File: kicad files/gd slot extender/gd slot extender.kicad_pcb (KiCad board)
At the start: 2 copper layers, 11 parts, among them J1 Card Edge, J2 Debug Header, J3 Sockety Socket Sock

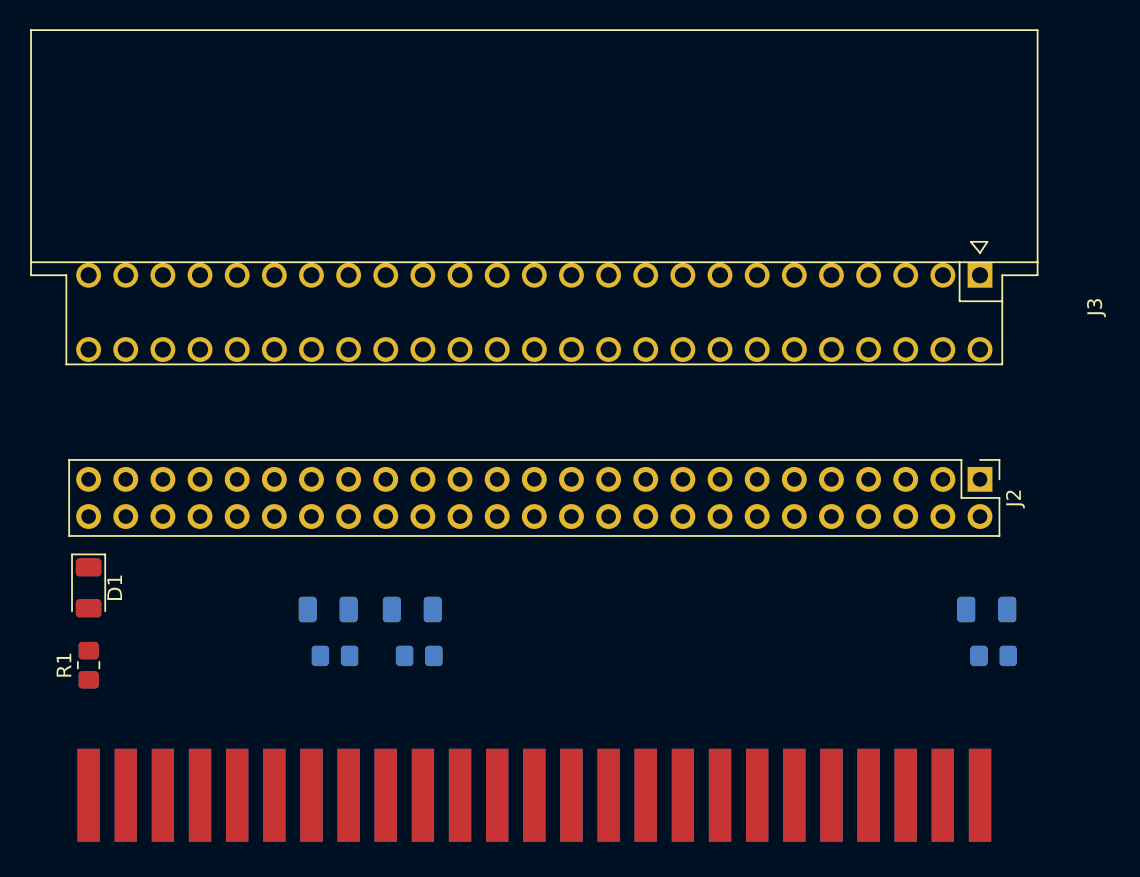
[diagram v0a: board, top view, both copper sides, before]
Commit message: rev1 ready for fab
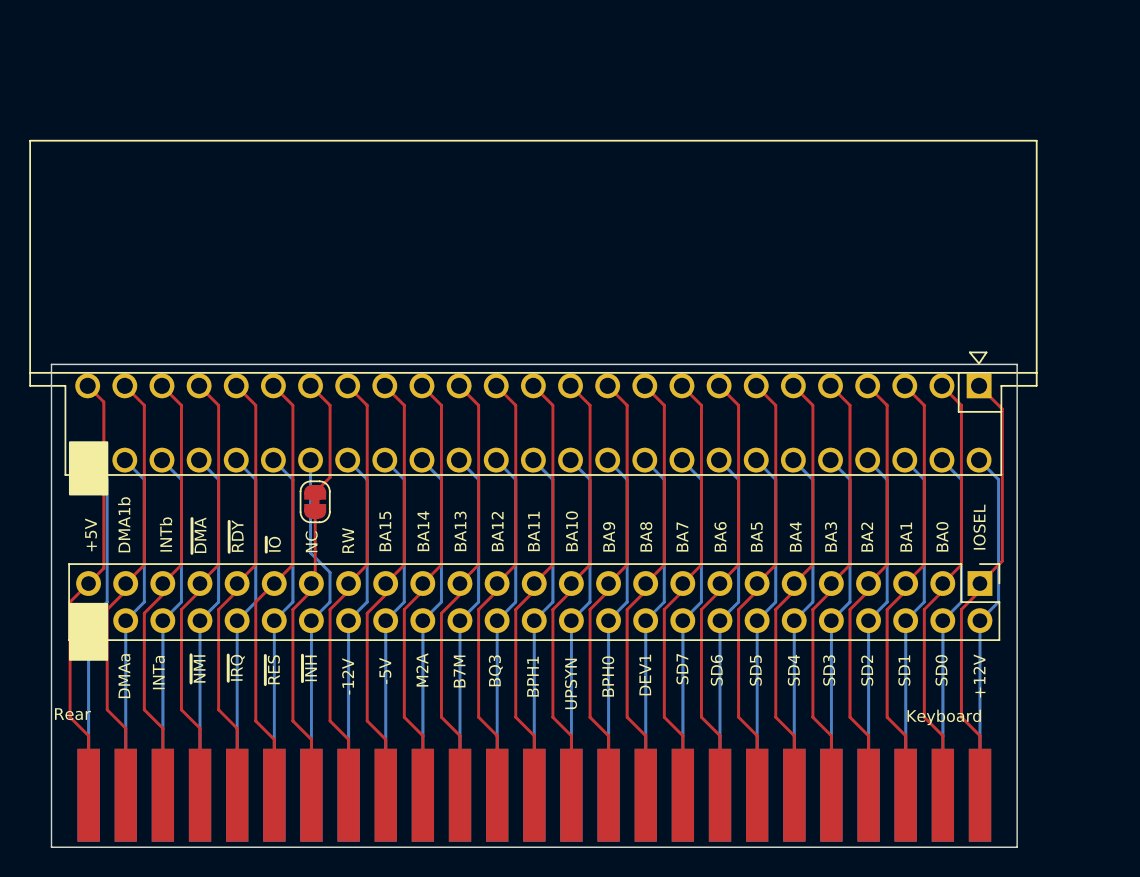
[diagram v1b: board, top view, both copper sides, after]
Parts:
- removed D1, D2, D3, D4: D_1206, LED_SMD:LED_1206_3216Metric
- removed R1, R2, R3, R4: 4k7, Resistor_SMD:R_0805_2012Metric_Pad1.20x1.40mm_HandSolder
- added JP1: Jumper_2_Bridged, Jumper:SolderJumper-2_P1.3mm_Bridged_RoundedPad1.0x1.5mm, F.Cu at (170.4, 106.9)
- moved J3 7.56 mm to (218.6, 102.1)
- moved J2 7.12 mm to (215.9, 112.5)
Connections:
- J1 pad 19: unconnected-(J1-Pad19) -> /NC
- J2 pad 19: unconnected-(J2-Pad19) -> /NC
- J3 pad 19: unconnected-(J3-Pad19) -> Net-(JP1-A)
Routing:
- net /~{IOSEL}: track 0.00 -> 30.3 mm
- net /~{DMA}: track 0.00 -> 30.1 mm
- net /RW: track 0.00 -> 30.1 mm
- net /BA9: track 0.00 -> 30.1 mm
- net /BA5: track 0.00 -> 30.1 mm
- net /BA2: track 0.00 -> 30.1 mm
- net /BA13: track 0.00 -> 30.1 mm
- net /~{RDY}: track 0.00 -> 30.1 mm
- net /BA15: track 0.00 -> 30.1 mm
- net /INTb: track 0.00 -> 30.1 mm
- net /BA8: track 0.00 -> 30.1 mm
- net /BA3: track 0.00 -> 30.1 mm
- net /BA12: track 0.00 -> 30.1 mm
- net /BA1: track 0.00 -> 30.1 mm
- net /BA7: track 0.00 -> 30.1 mm
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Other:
- board outline added: 66 x 33 mm
- board text added: "+12V"
- board text added: "+5V"
- board text added: "-12V"
- board text added: "-5V"
- board text added: "B7M"
- board text added: "BA0"
- board text added: "BA1"
- board text added: "BA10"
- board text added: "BA11"
- board text added: "BA12"
- board text added: "BA13"
- board text added: "BA14"
- board text added: "BA15"
- board text added: "BA2"
- board text added: "BA3"
- board text added: "BA4"
- board text added: "BA5"
- board text added: "BA6"
- board text added: "BA7"
- board text added: "BA8"
- board text added: "BA9"
- board text added: "BPH0"
- board text added: "BPH1"
- board text added: "BQ3"
- board text added: "DEV1"
- board text added: "DMA1b"
- board text added: "DMAa"
- board text added: "INTa"
- board text added: "INTb"
- board text added: "IOSEL"
- board text added: "Keyboard"
- board text added: "M2A"
- board text added: "NC"
- board text added: "RW"
- board text added: "Rear"
- board text added: "SD0"
- board text added: "SD1"
- board text added: "SD2"
- board text added: "SD3"
- board text added: "SD4"
- board text added: "SD5"
- board text added: "SD6"
- board text added: "SD7"
- board text added: "UPSYN"
- board text added: "gd slot exp, rev1, @baldengineer"
- board text added: "~{DMA}"
- board text added: "~{INH}"
- board text added: "~{IO}"
- board text added: "~{IRQ}"
- board text added: "~{NMI}"
- board text added: "~{RDY}"
- board text added: "~{RES}"
